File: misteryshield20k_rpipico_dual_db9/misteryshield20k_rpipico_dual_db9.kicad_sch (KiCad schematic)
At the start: 56 parts, among them J1 Joystick, J2 Joystick, J3 USB_C_Receptacle_PowerOnly, J4 Conn_01x20_Pin, J5 Conn_01x02_Pin, J7 Conn_01x20_Pin, Q1 2N7002, Q10 2N7002, Q11 2N7002, Q12 2N7002, Q2 2N7002, Q3 2N7002, Q4 2N7002, Q5 2N7002, Q6 2N7002, Q7 2N7002, Q8 2N7002, Q9 2N7002

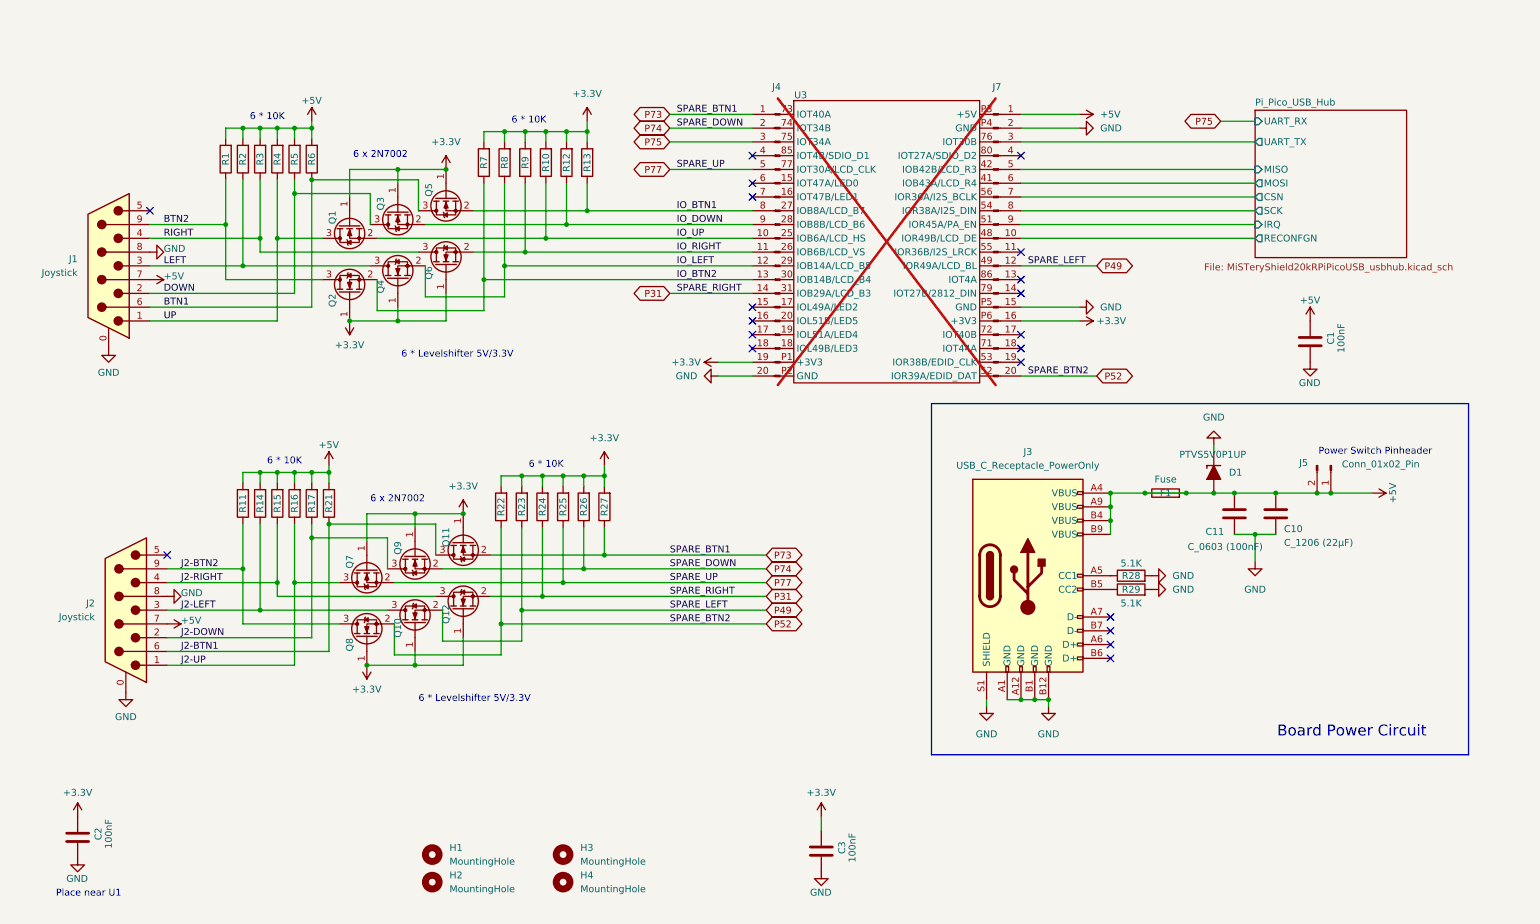
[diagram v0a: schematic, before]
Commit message: Add files via upload
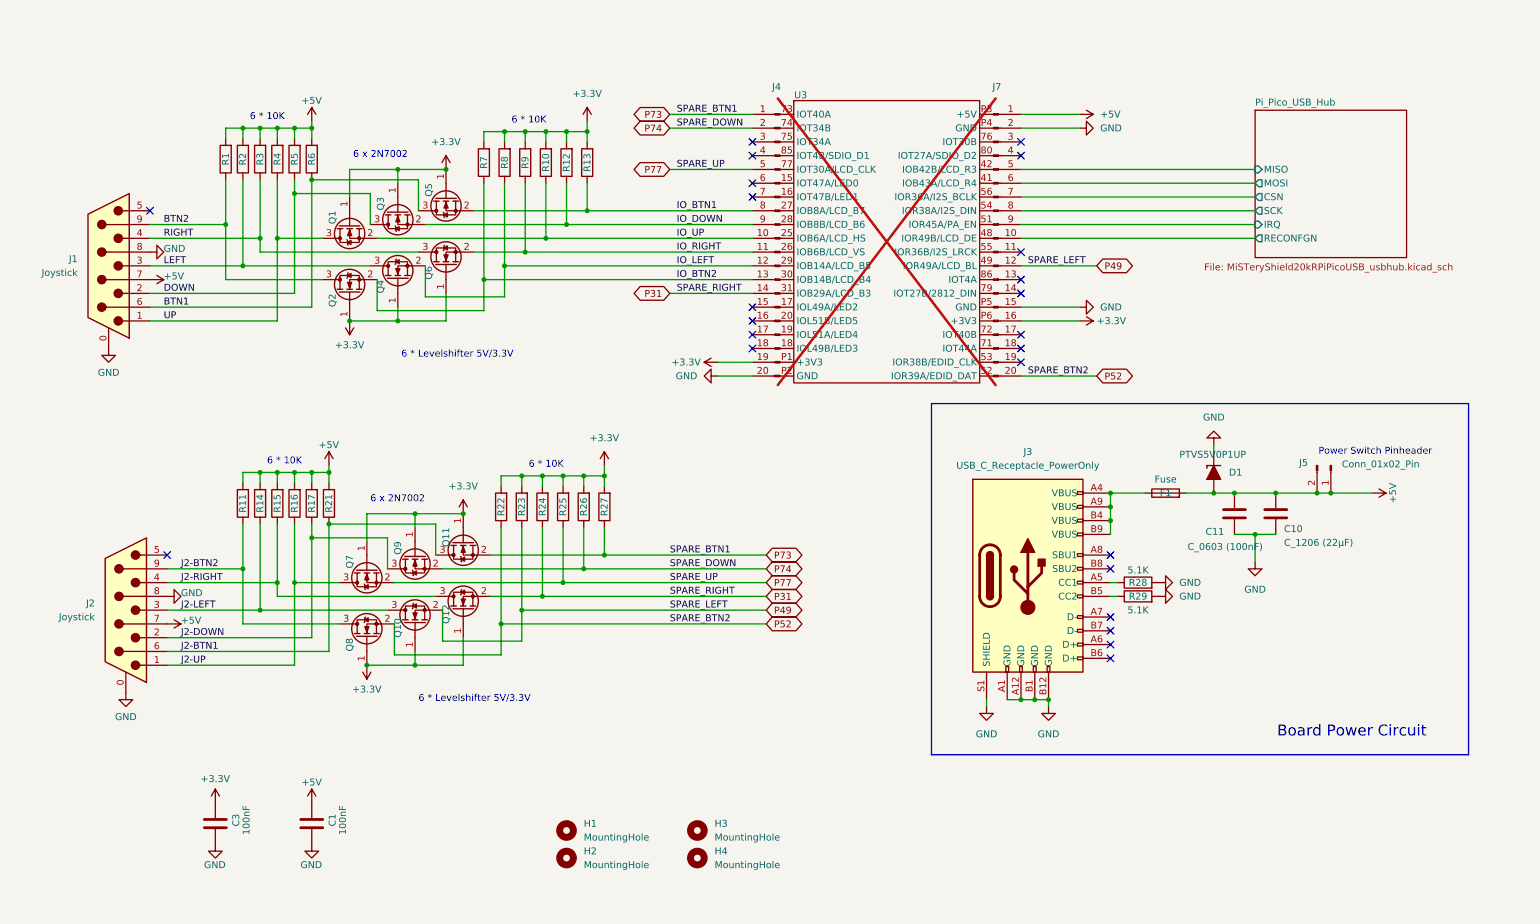
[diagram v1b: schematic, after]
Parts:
- removed C2: 100nF, Capacitor_SMD:C_0805_2012Metric, symbol Device:C
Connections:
- net +5V: no longer F1.1, J3.A4 (VBUS), J3.A9 (VBUS), J3.B4 (VBUS), J3.B9 (VBUS)
- net P75: no longer names the net of J4.3 (Pin_3)
- net Pi_Pico_USB_Hub/UART_TX: no longer names the net of J7.3 (Pin_3)
- new net: F1.1, J3.A4 (VBUS), J3.A9 (VBUS), J3.B4 (VBUS), J3.B9 (VBUS)
- no-connect marks 20 -> 24
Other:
- sheet Pi_Pico_USB_Hub ports: added none; removed UART_RX, UART_TX
- note removed: "Place near U1"
- moved on the sheet: C1, C3, H1, H2, H3, H4, R28, R29

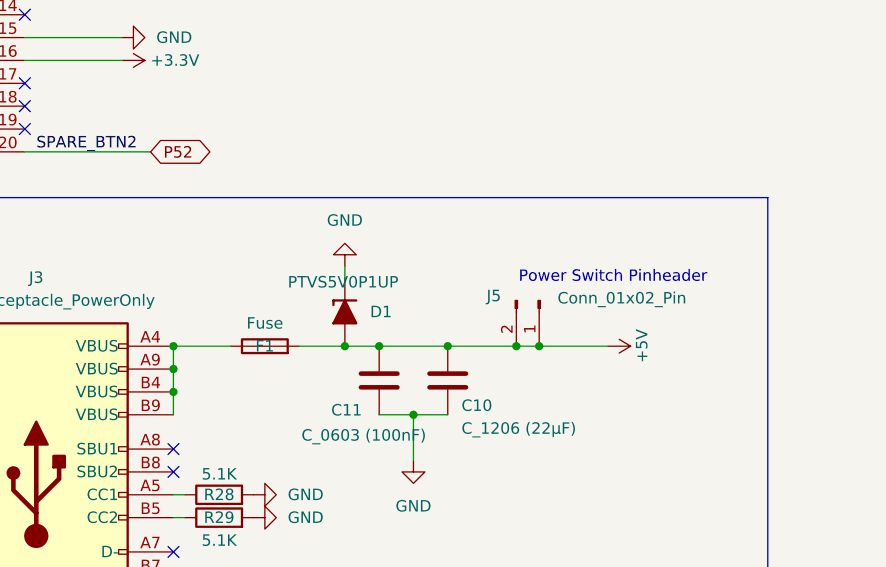
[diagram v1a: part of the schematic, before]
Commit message: Add files via upload
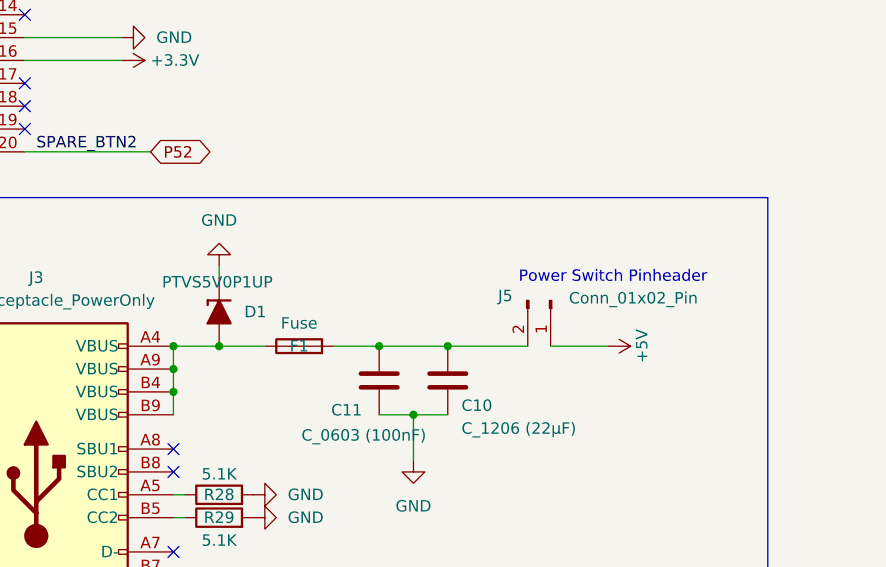
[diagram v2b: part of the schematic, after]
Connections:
- net +5V: no longer C10.1, C11.1, D1.2 (A), F1.2, J5.2 (Pin_2)
- net at F1.1, J3.A4 (VBUS), J3.A9 (VBUS)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: now also D1.2 (A)
- new net: C10.1, C11.1, F1.2, J5.2 (Pin_2)
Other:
- moved on the sheet: D1, F1, J5
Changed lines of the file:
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@@
 	)
 	(junction
-		(at 254 114.3)
-		(diameter 0)
-		(color 0 0 0 0)
-	)
-	(junction
 		(at 71.755 110.49)
 		(diameter 0)
@@
 	)
 	(junction
-		(at 234.95 114.3)
-		(diameter 0)
-		(color 0 0 0 0)
-	)
-	(junction
 		(at 100.33 74.93)
 		(diameter 0)
@@
 	)
 	(junction
-		(at 111.76 47.625)
+		(at 220.98 114.3)
 		(diameter 0)
 		(color 0 0 0 0)
 	)
 	(junction
-		(at 256.54 114.3)
+		(at 111.76 47.625)
 		(diameter 0)
 		(color 0 0 0 0)
@@
 	(wire
 		(pts
+			(xy 257.81 114.3) (xy 264.16 114.3)
+		)
+		(stroke
+			(width 0)
+			(type default)
+		)
+	)
+	(wire
+		(pts
 			(xy 201.93 152.4) (xy 199.39 152.4)
 		)
@@
 	(wire
 		(pts
-			(xy 246.38 114.3) (xy 254 114.3)
+			(xy 246.38 114.3) (xy 255.27 114.3)
 		)
 		(stroke
@@
 	(wire
 		(pts
-			(xy 256.54 114.3) (xy 264.16 114.3)
-		)
-		(stroke
-			(width 0)
-			(type default)
-		)
-	)
-	(wire
-		(pts
-			(xy 234.95 105.41) (xy 234.95 106.68)
+			(xy 220.98 105.41) (xy 220.98 106.68)
 		)
 		(stroke
@@
 	(wire
 		(pts
+			(xy 233.68 114.3) (xy 238.76 114.3)
+		)
+		(stroke
+			(width 0)
+			(type default)
+		)
+	)
+	(wire
+		(pts
 			(xy 71.755 110.49) (xy 71.755 109.22)
 		)
@@
 	(wire
 		(pts
-			(xy 254 114.3) (xy 256.54 114.3)
-		)
-		(stroke
-			(width 0)
-			(type default)
-		)
-	)
-	(wire
-		(pts
-			(xy 215.9 114.3) (xy 222.25 114.3)
+			(xy 215.9 114.3) (xy 220.98 114.3)
 		)
 		(stroke
@@
 	(wire
 		(pts
-			(xy 234.95 114.3) (xy 238.76 114.3)
-		)
-		(stroke
-			(width 0)
-			(type default)
-		)
-	)
-	(wire
-		(pts
 			(xy 101.6 125.73) (xy 122.555 125.73)
 		)
@@
 	(wire
 		(pts
-			(xy 118.745 111.125) (xy 122.555 111.125)
+			(xy 220.98 114.3) (xy 226.06 114.3)
 		)
 		(stroke
@@
 	(wire
 		(pts
-			(xy 59.055 67.31) (xy 59.055 56.515)
+			(xy 118.745 111.125) (xy 122.555 111.125)
 		)
 		(stroke
@@
 	(wire
 		(pts
-			(xy 199.39 80.01) (xy 210.185 80.01)
+			(xy 59.055 67.31) (xy 59.055 56.515)
 		)
 		(stroke
@@
 	(wire
 		(pts
-			(xy 229.87 114.3) (xy 234.95 114.3)
+			(xy 199.39 80.01) (xy 210.185 80.01)
 		)
 		(stroke
@@
 	(symbol
 		(lib_id "PCM_Diode_TVS_AKL:PTVS5V0P1UP")
-		(at 234.95 110.49 90)
+		(at 220.98 110.49 90)
 		(unit 1)
 		(exclude_from_sim no)
@@
 		(dnp no)
 		(property "Reference" "D1"
-			(at 237.744 110.49 90)
+			(at 223.774 110.49 90)
 			(effects
 				(font
@@
 		)
 		(property "Value" "PTVS5V0P1UP"
-			(at 228.6 107.188 90)
+			(at 214.63 107.188 90)
 			(effects
 				(font
@@
 		)
 		(property "Footprint" "Diode_SMD:D_SOD-123"
-			(at 234.95 110.49 0)
+			(at 220.98 110.49 0)
 			(effects
 				(font
@@
 		)
 		(property "Datasheet" "https://www.tme.eu/Document/475226a1f5f23e88222b181b564f5c39/PTVSXP1UP_SER.pdf"
-			(at 234.95 110.49 0)
+			(at 220.98 110.49 0)
 			(effects
 				(font
@@
 		)
 		(property "Description" "SOD-128 Unidirectional TVS diode, 5V, 600W, Alternate KiCAD Library"
-			(at 234.95 110.49 0)
+			(at 220.98 110.49 0)
 			(effects
 				(font
@@
 	(symbol
 		(lib_id "power:GND")
-		(at 234.95 105.41 180)
+		(at 220.98 105.41 180)
 		(unit 1)
 		(exclude_from_sim no)
@@
 		(fields_autoplaced yes)
 		(property "Reference" "#PWR033"
-			(at 234.95 99.06 0)
+			(at 220.98 99.06 0)
 			(effects
 				(font
@@
 		)
 		(property "Value" "GND"
-			(at 234.95 100.33 0)
+			(at 220.98 100.33 0)
 			(effects
 				(font
@@
 		)
 		(property "Footprint" ""
-			(at 234.95 105.41 0)
+			(at 220.98 105.41 0)
 			(effects
 				(font
@@
 		)
 		(property "Datasheet" ""
-			(at 234.95 105.41 0)
+			(at 220.98 105.41 0)
 			(effects
 				(font
@@
 		)
 		(property "Description" ""
-			(at 234.95 105.41 0)
+			(at 220.98 105.41 0)
 			(effects
 				(font
@@
 	(symbol
 		(lib_id "Device:Fuse")
-		(at 226.06 114.3 90)
+		(at 229.87 114.3 90)
 		(unit 1)
 		(exclude_from_sim no)
@@
 		(dnp no)
 		(property "Reference" "F1"
-			(at 226.06 114.3 90)
+			(at 229.87 114.3 90)
 			(effects
 				(font
@@
 		)
 		(property "Value" "Fuse"
-			(at 226.06 111.76 90)
+			(at 229.87 111.76 90)
 			(effects
 				(font
@@
 		)
 		(property "Footprint" "Fuse:Fuse_1812_4532Metric"
-			(at 226.06 116.078 90)
+			(at 229.87 116.078 90)
 			(effects
 				(font
@@
 		)
 		(property "Datasheet" "~"
-			(at 226.06 114.3 0)
+			(at 229.87 114.3 0)
 			(effects
 				(font
@@
 		)
 		(property "Description" "Polyfuse"
-			(at 226.06 117.094 90)
+			(at 229.87 117.094 90)
 			(effects
 				(font
@@
 		)
 		(instances
-			(project ""
+			(project "misteryshield20k_rpipico_dual_db9"
 				(path "/18b63fd5-4a6d-47a9-b0d3-ab759ce46098"
 					(reference "F1")
@@
 	(symbol
 		(lib_id "Connector:Conn_01x02_Pin")
-		(at 256.54 109.22 270)
+		(at 257.81 109.22 270)
 		(unit 1)
 		(exclude_from_sim no)
@@
 		(dnp no)
 		(property "Reference" "J5"
-			(at 250.698 108.712 90)
+			(at 251.968 108.712 90)
 			(effects
 				(font
@@
 		)
 		(property "Value" "Conn_01x02_Pin"
-			(at 258.572 108.966 90)
+			(at 259.842 108.966 90)
 			(effects
 				(font
@@
 		)
 		(property "Footprint" "Connector_PinHeader_2.54mm:PinHeader_1x02_P2.54mm_Horizontal"
-			(at 256.54 109.22 0)
+			(at 257.81 109.22 0)
 			(effects
 				(font
@@
 		)
 		(property "Datasheet" "~"
-			(at 256.54 109.22 0)
+			(at 257.81 109.22 0)
 			(effects
 				(font
@@
 		)
 		(property "Description" "Generic connector, single row, 01x02, script generated"
-			(at 256.54 109.22 0)
+			(at 257.81 109.22 0)
 			(effects
 				(font
@@
 		)
 		(instances
-			(project ""
+			(project "misteryshield20k_rpipico_dual_db9"
 				(path "/18b63fd5-4a6d-47a9-b0d3-ab759ce46098"
 					(reference "J5")

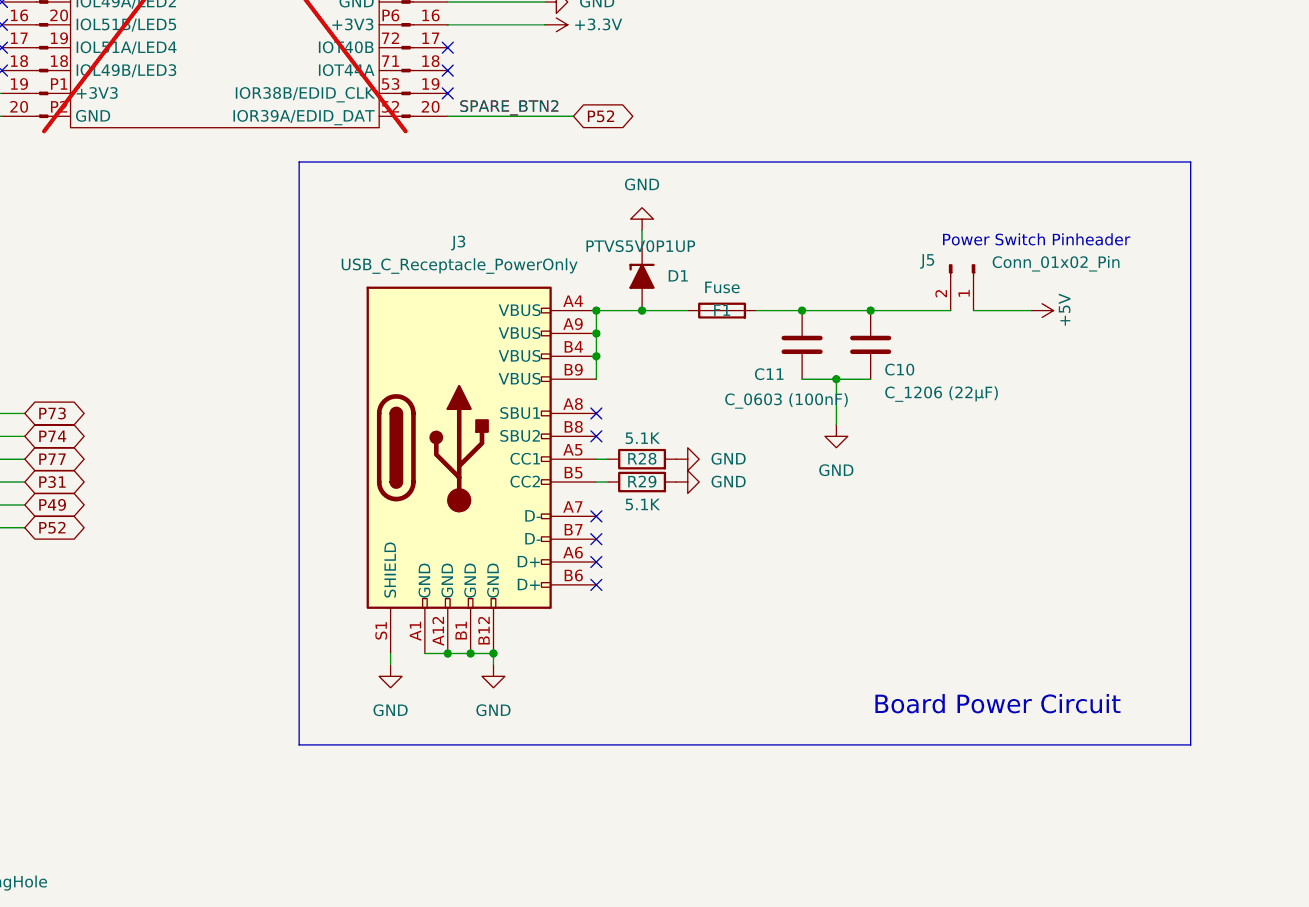
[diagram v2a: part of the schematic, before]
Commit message: Add files via upload
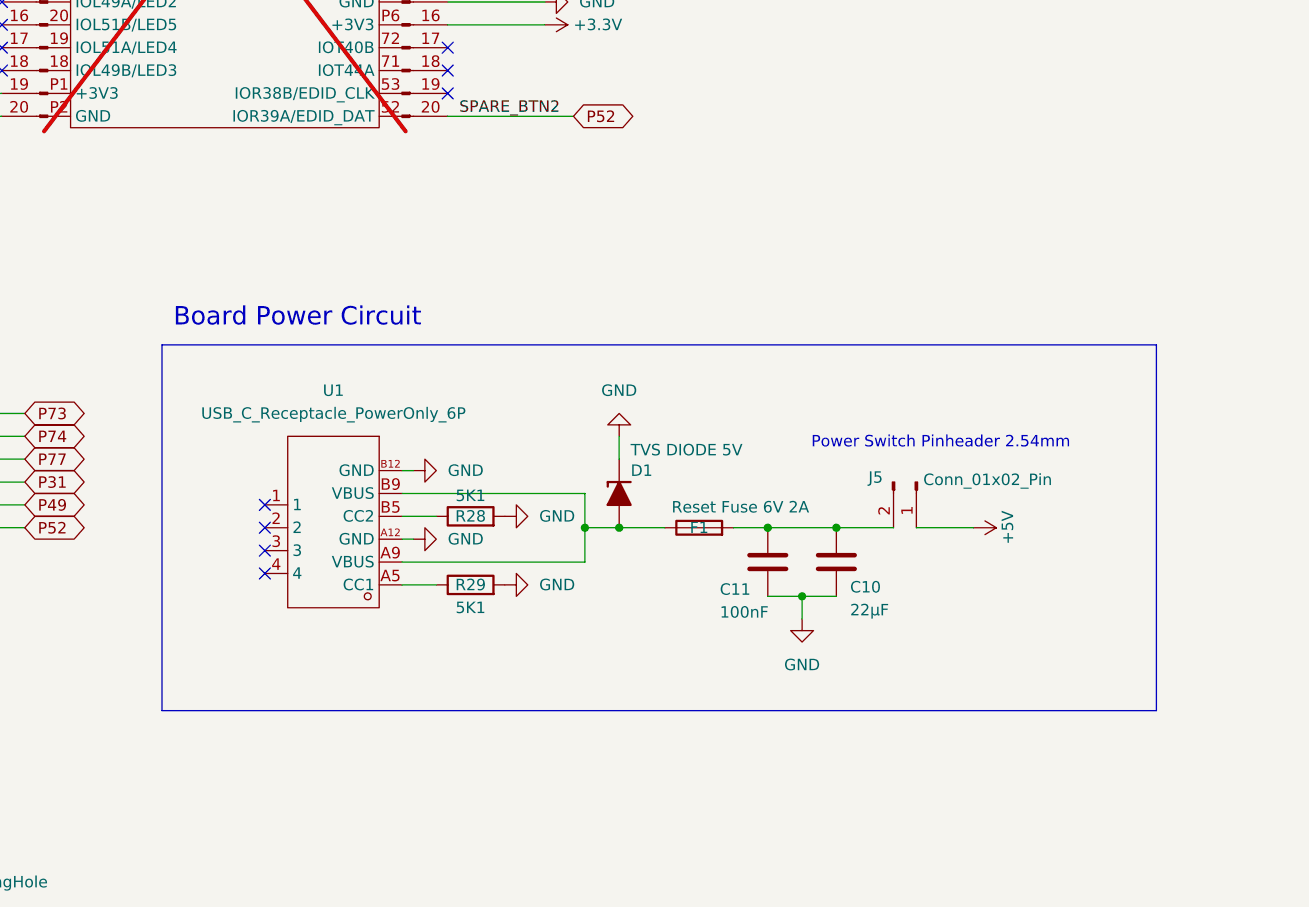
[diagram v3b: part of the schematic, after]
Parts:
- removed J3: USB_C_Receptacle_PowerOnly, Connector_USB:USB_C_Receptacle_GCT_USB4085, symbol Connector:USB_C_Receptacle_USB2.0_14P
- added U1: USB_C_Receptacle_PowerOnly_6P, TYPE-C-SMD_XUNPU_TYPEC-250C-BRP6, symbol Geralds_Library:TYPEC-250C-BRP6
- C10: value C_1206 (22µF) -> 22µF; footprint PCM_Capacitor_SMD_AKL:C_1206_3216Metric -> Capacitor_SMD:C_0805_2012Metric; LCSC Part # (none) -> C45783
- C11: value C_0603 (100nF) -> 100nF; footprint PCM_Capacitor_SMD_AKL:C_0603_1608Metric -> Capacitor_SMD:C_0805_2012Metric; LCSC Part # (none) -> C49678
- D1: value PTVS5V0P1UP -> TVS DIODE 5V; Bemerkung (none) -> PTVS5V0P1UP; LCSC Part # (none) -> C426873
- F1: value Fuse -> Reset Fuse 6V 2A; footprint Fuse:Fuse_1812_4532Metric -> Fuse:Fuse_0805_2012Metric; JLCPCB Part # (none) -> C70158
- R28, R29: value 5.1K -> 5K1; footprint Resistor_SMD:R_0603_1608Metric -> Resistor_SMD:R_0805_2012Metric
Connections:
- net GND: now also U1.A12 (GND), U1.B12 (GND)
- net at D1.2 (A), F1.1: now also U1.A9 (VBUS), U1.B9 (VBUS)
- net at R29.1: now also U1.A5 (CC1)
- net at R28.1: now also U1.B5 (CC2)
- no-connect marks 24 -> 22
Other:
- note added: "Power Switch Pinheader 2.54mm"
- note removed: "Power Switch Pinheader"
- moved on the sheet: C10, C11, D1, F1, J5, R28, R29

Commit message: Add files via upload
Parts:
- D1: footprint Diode_SMD:D_SOD-123 -> MiSTeryShield20kRPiPico:SOD-128_L3.7-W2.5-LS4.7-RD; JLCPCB Part # (none) -> C426873; LCSC Part # C426873 -> (none)
- J5: JLCPCB Part # (none) -> C492410
- U1: JLCPCB Part # (none) -> C5374812; Supplier Part C5374812 -> (none)
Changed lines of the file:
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@@
 			)
 		)
-		(property "Footprint" "Diode_SMD:D_SOD-123"
+		(property "Footprint" "MiSTeryShield20kRPiPico:SOD-128_L3.7-W2.5-LS4.7-RD"
 			(at 218.44 134.62 0)
 			(effects
@@
 			)
 		)
-		(property "LCSC Part #" "C426873"
+		(property "JLCPCB Part #" "C426873"
 			(at 218.44 134.62 90)
 			(effects
@@
 			)
 		)
-		(property "Supplier Part" "C5374812"
+		(property "Supplier" "LCSC"
 			(at 186.69 137.16 0)
 			(effects
@@
 			)
 		)
-		(property "Supplier" "LCSC"
+		(property "LCSC Part Name" "Type-C 母 卧贴"
 			(at 186.69 137.16 0)
 			(effects
@@
 			)
 		)
-		(property "LCSC Part Name" "Type-C 母 卧贴"
+		(property "JLCPCB Part #" "C5374812"
 			(at 186.69 137.16 0)
 			(effects
@@
 			(at 251.46 133.35 0)
 			(effects
+				(font
+					(size 1.27 1.27)
+				)
+				(hide yes)
+			)
+		)
+		(property "JLCPCB Part #" "C492410"
+			(at 251.46 133.35 0)
+			(effects
